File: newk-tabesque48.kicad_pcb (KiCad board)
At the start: 2 copper layers, 192.5 x 118.4 mm, 98 parts, among them SW1 SW_Push, U1 ProMicro

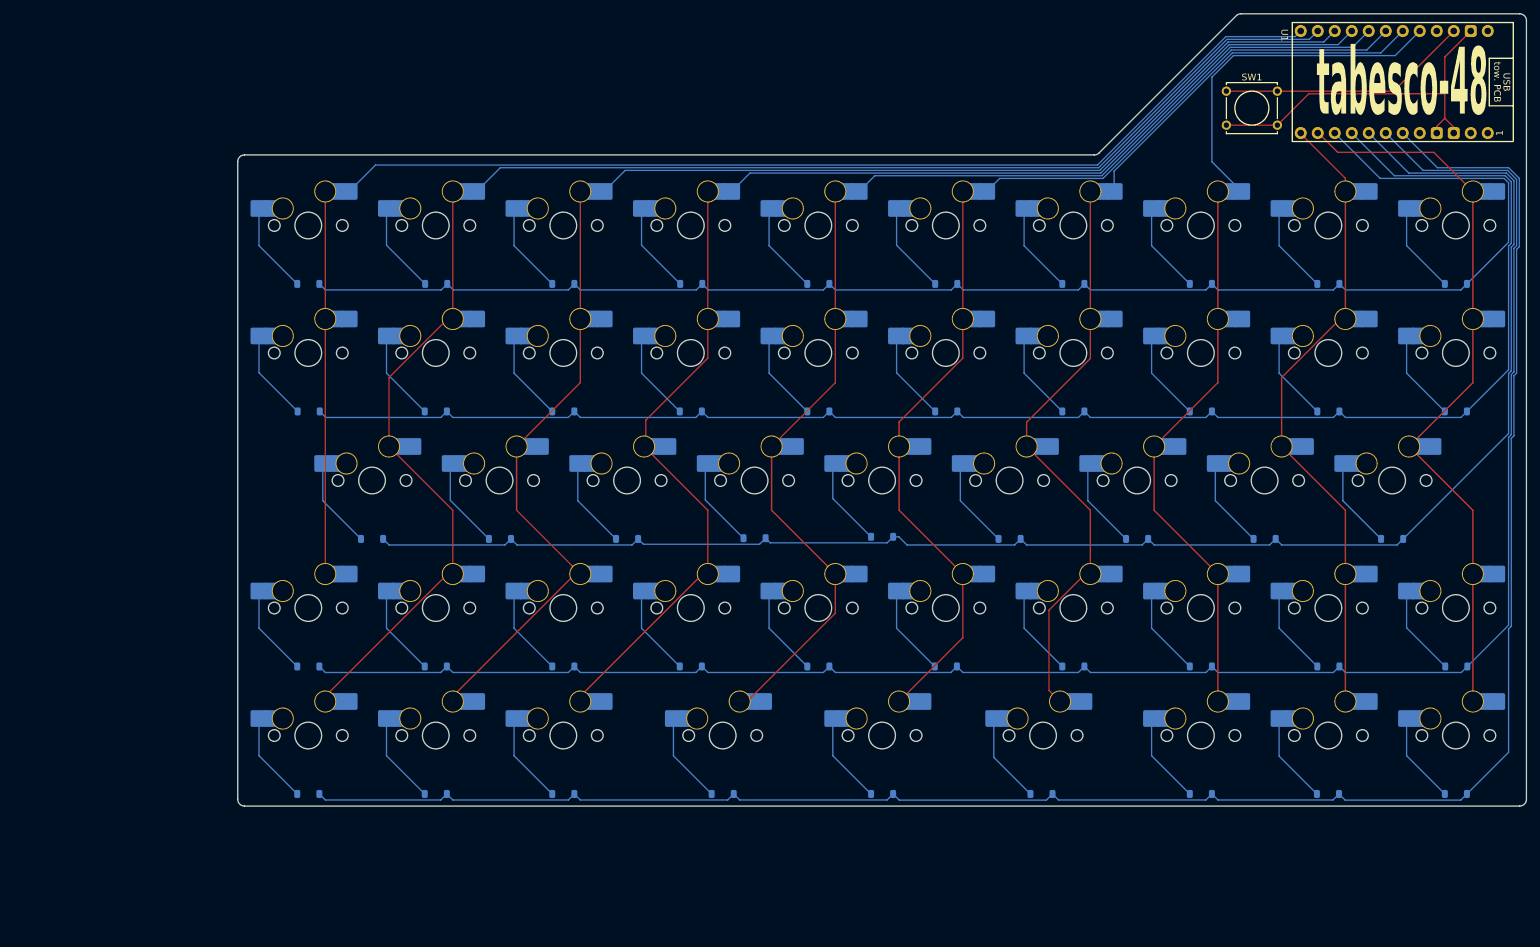
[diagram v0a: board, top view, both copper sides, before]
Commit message: created tabasco slide verson
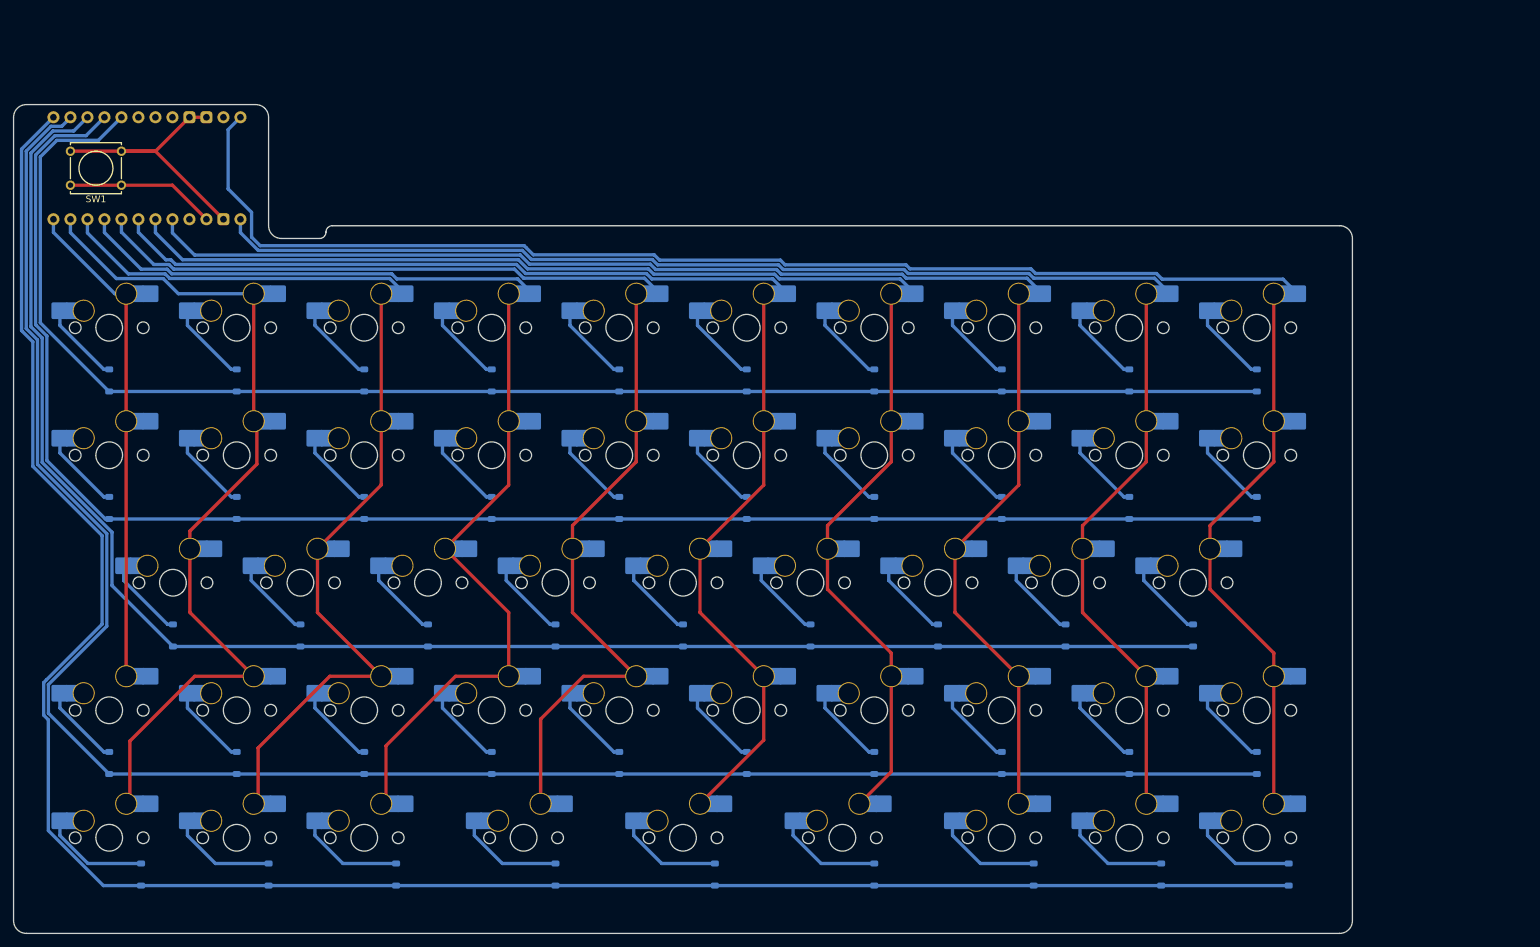
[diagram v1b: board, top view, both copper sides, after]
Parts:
- U1: moved to B.Cu
- moved U1 186.8 mm to (45.4, 49.4), turned to 90 degrees
- moved SW1 165.7 mm to (41.6, 51.9), turned to 180 degrees
- moved MX43 33.6 mm to (149.3, 149.4)
- moved MX1 33.4 mm to (211.2, 73.2)
- moved MX11 33.4 mm to (211.2, 92.2)
- moved MX12 33.4 mm to (192.1, 92.2)
- moved MX14 33.4 mm to (154.0, 92.2)
- moved MX15 33.4 mm to (135.0, 92.2)
- moved MX16 33.4 mm to (115.9, 92.2)
- moved MX17 33.4 mm to (96.9, 92.2)
- moved MX18 33.4 mm to (77.8, 92.2)
- moved MX19 33.4 mm to (58.8, 92.2)
- moved MX2 33.4 mm to (192.1, 73.2)
- moved MX21 33.4 mm to (201.6, 111.3)
- moved MX22 33.4 mm to (182.6, 111.3)
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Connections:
- U1 pad 1: unconnected-(U1-D3-TX-Pad1) -> /col0
- U1 pad 10: /row0 -> /row2
- U1 pad 11: /col0 -> /row3
- U1 pad 12: /col1 -> /row4
- U1 pad 13: unconnected-(U1-B0-Pad13) -> /col1
- U1 pad 5: /col_tmo -> unconnected-(U1-D1-Pad5)
- U1 pad 6: /row4 -> unconnected-(U1-D0-Pad6)
- U1 pad 7: /row3 -> unconnected-(U1-D4-Pad7)
- U1 pad 8: /row2 -> /row0
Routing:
- net /col0: track 111.3 -> 264.0 mm
- net /col1: track 96.1 -> 228.7 mm
- net /col9: track 209.3 -> 77.3 mm
- net /col8: track 228.5 -> 134.2 mm
- net /col2: track 136.9 -> 219.9 mm
- net /col3: track 142.6 -> 205.3 mm
- net /col7: track 211.5 -> 149.7 mm
- net /col4: track 157.6 -> 190.8 mm
- net /col6: track 195.2 -> 166.4 mm
- net RST: track 37.7 -> 22.4 mm
- net /row4: track 292.9 -> 306.1 mm
- net GND: track 54.7 -> 41.9 mm
- net /row3: track 276.5 -> 285.6 mm
- net /col5: track 176.7 -> 180.8 mm
- net Net-(D43-A): track 13.5 -> 16.1 mm
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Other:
- board size 192.5 x 118.4 mm -> 200 x 123.8 mm
- board text removed: "tabesco-48"
